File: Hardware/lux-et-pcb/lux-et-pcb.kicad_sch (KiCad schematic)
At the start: 98 parts, among them J1 Conn_01x03_Socket, J2 Conn_01x03_Socket, J3 Conn_01x03_Socket, J4 USB_C_Receptacle_PowerOnly_6P, Q1 PMOS, Q2 PMOS, Q3 AO3400A, Q4 AO3400A, Q5 AO3400A, Q6 2N7002K, Q7 2N7002K, U1 XL1509-5V, U2 AP2112K-3.3, U3 ESP32-WROOM-32, U4 TP4056

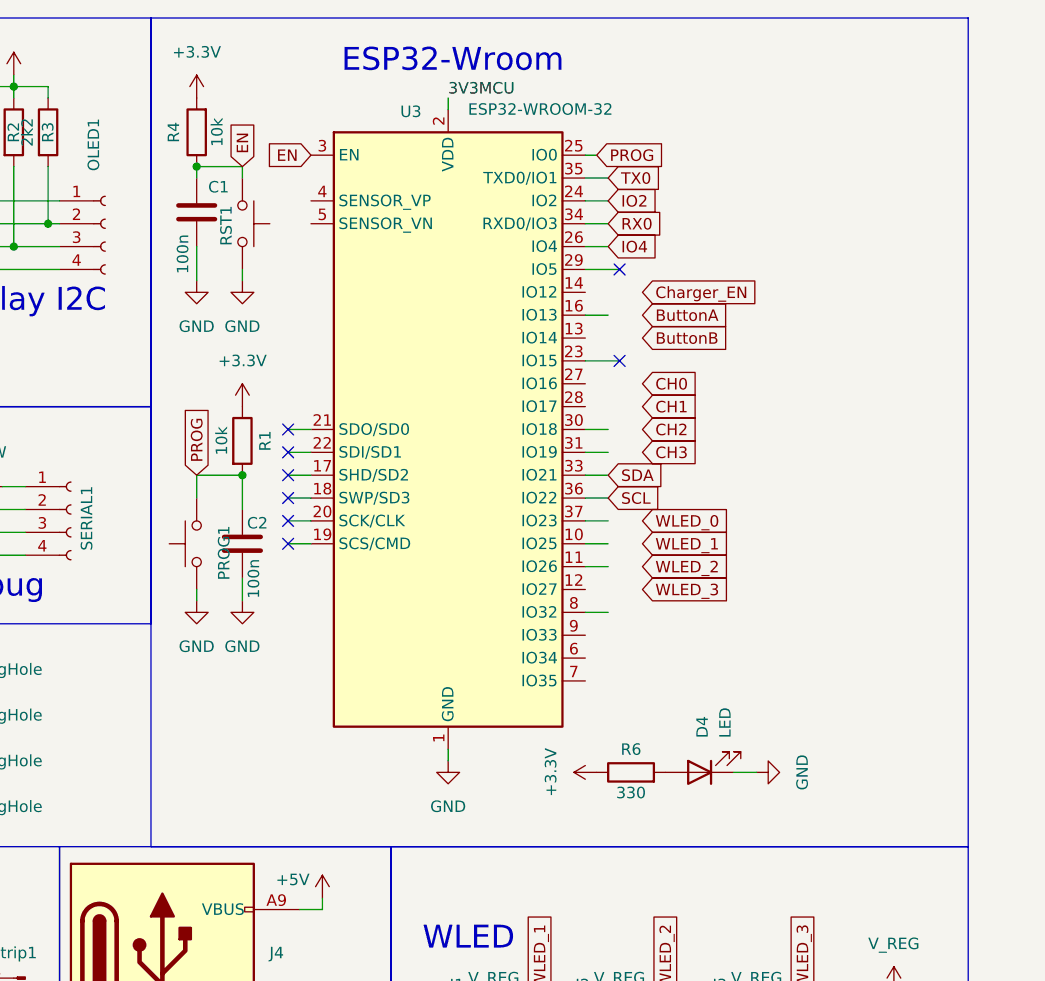
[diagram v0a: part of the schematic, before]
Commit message: Minor update
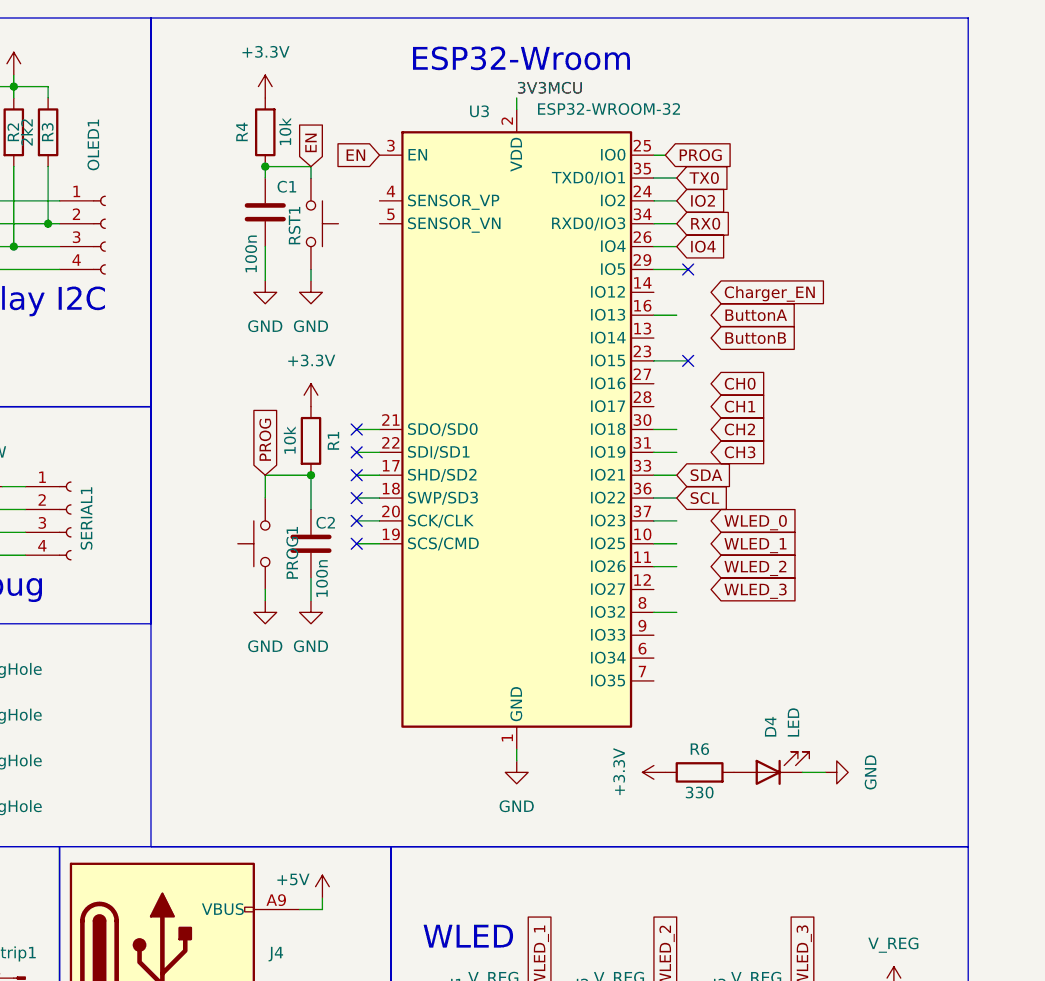
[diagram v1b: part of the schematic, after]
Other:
- moved on the sheet: C1, C2, D4, PROG1, R1, R4, R6, RST1, U3
